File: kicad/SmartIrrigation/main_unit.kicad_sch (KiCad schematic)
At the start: 20 parts, among them J1 RJ45, J2 RJ45, J3 RJ45, J4 RJ45, J5 RJ45, J6 RJ45, J7 Micro_SD_Card, J7 RJ45, J8 RJ45, U6 MT3608

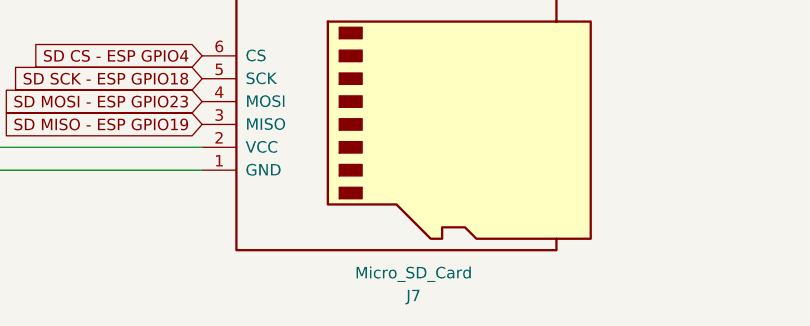
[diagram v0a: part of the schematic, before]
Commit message: added schematics images
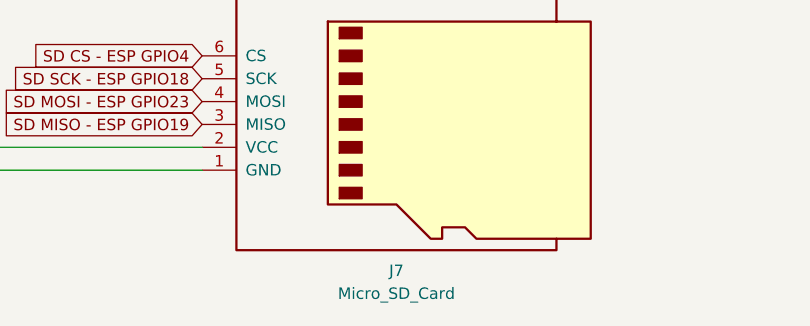
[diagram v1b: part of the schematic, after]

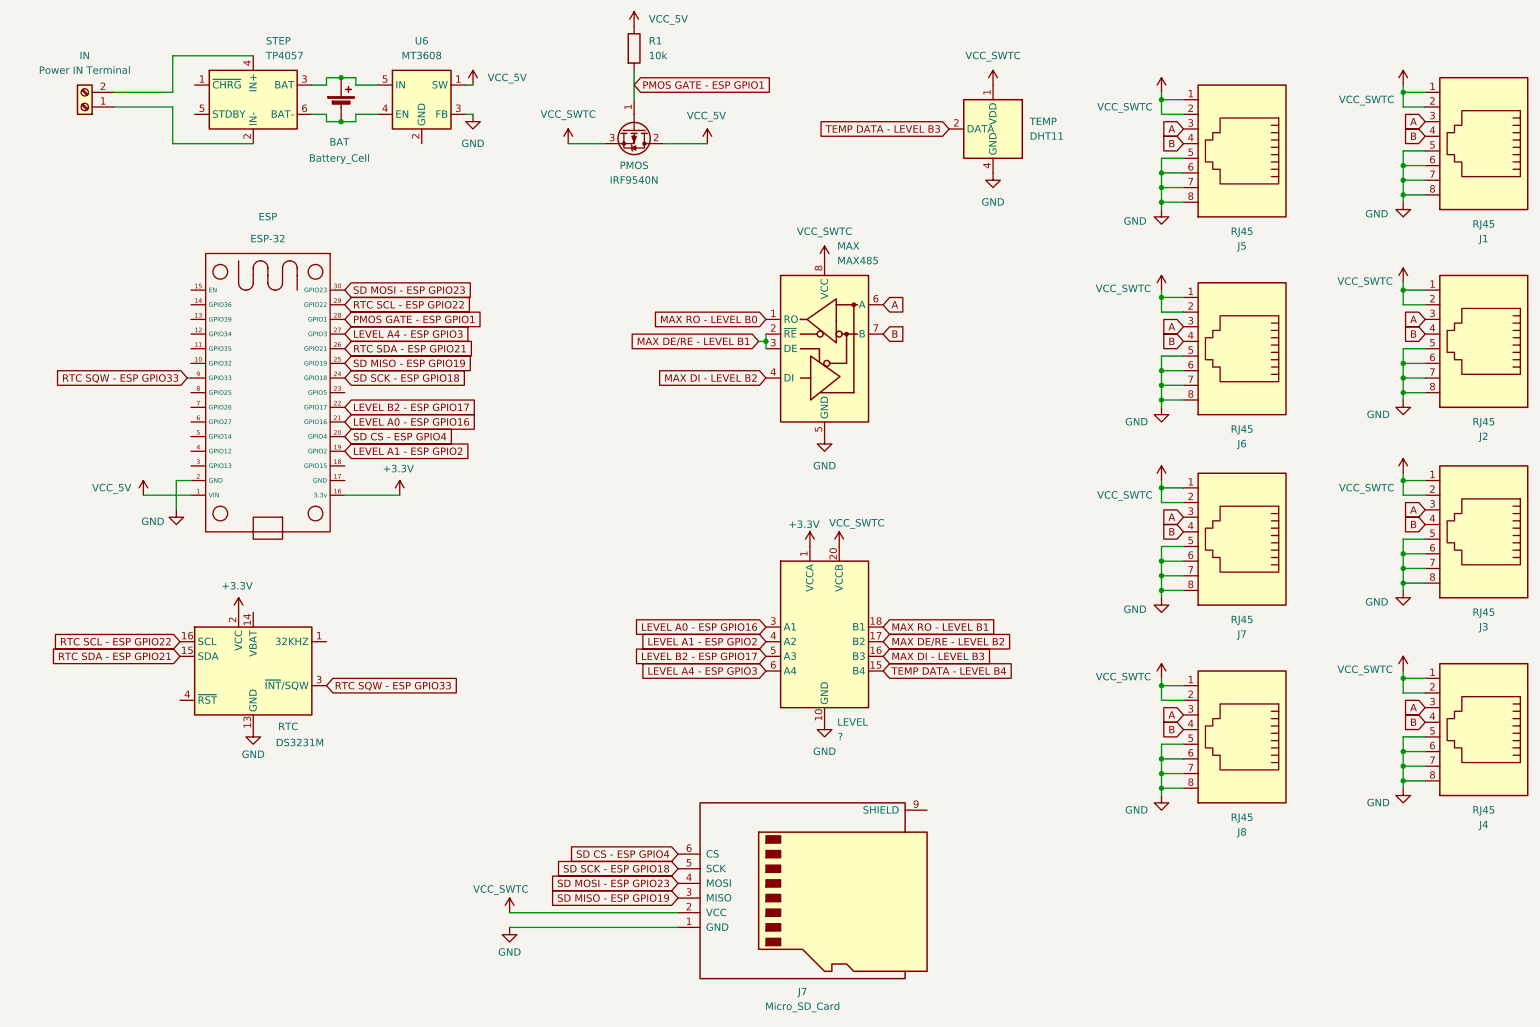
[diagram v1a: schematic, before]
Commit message: new schemes
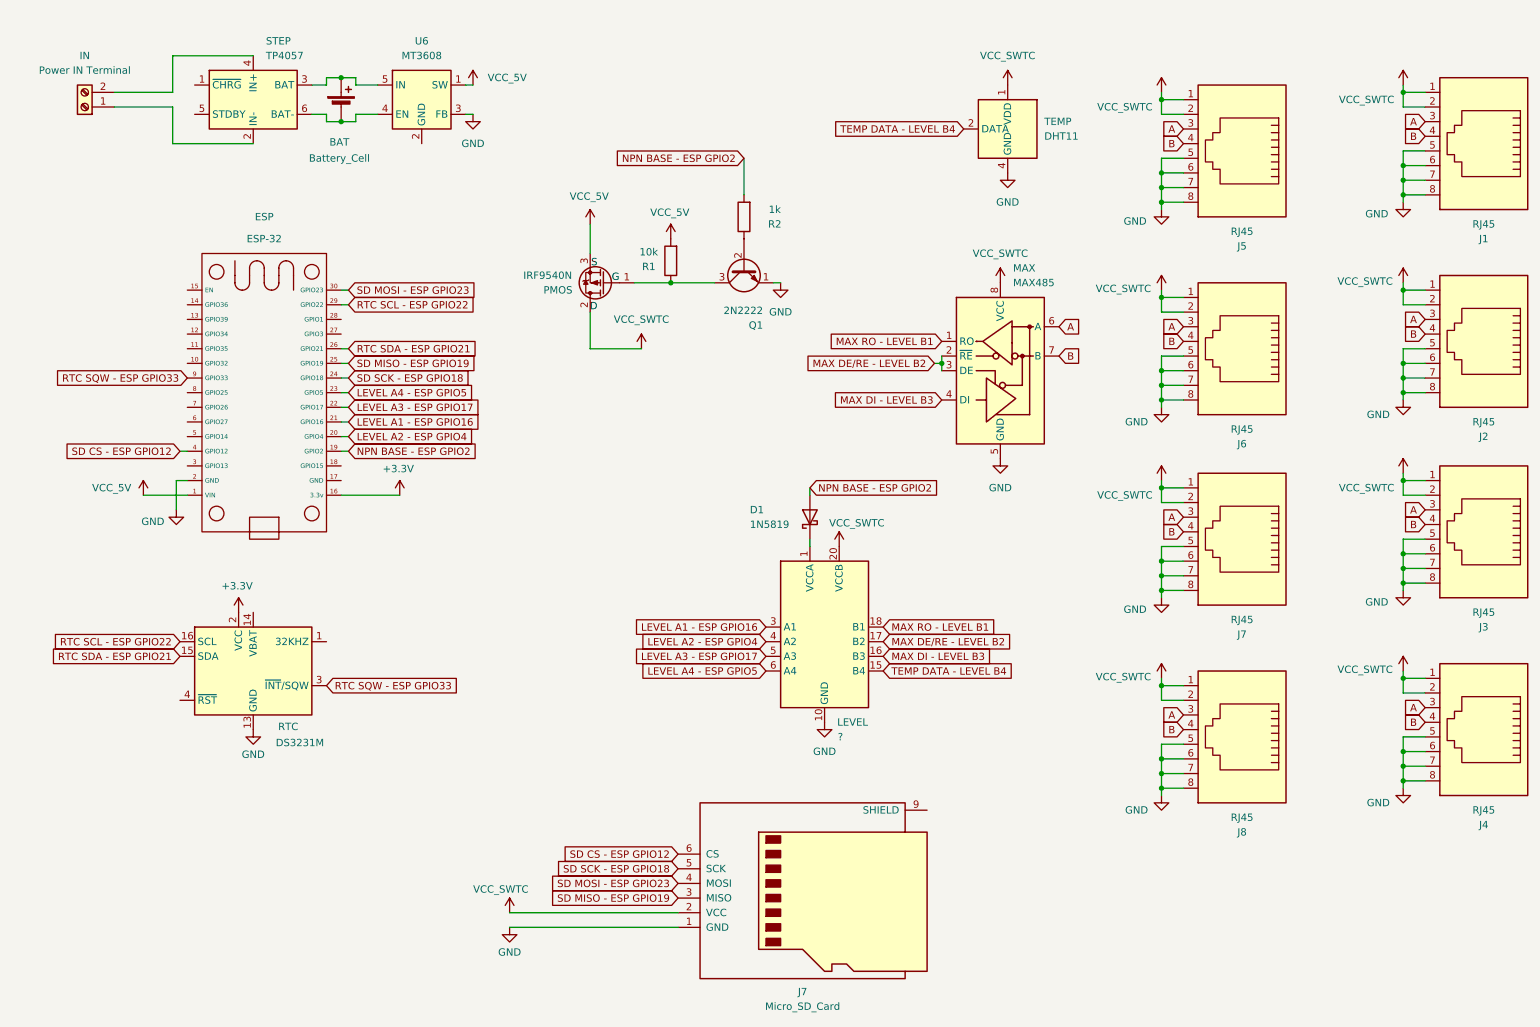
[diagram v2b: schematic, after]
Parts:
- added D1: 1N5819, Diode_THT:D_DO-41_SOD81_P10.16mm_Horizontal, symbol Diode:1N5819
- added Q1: 2N2222, Package_TO_SOT_THT:TO-39-3, symbol Transistor_BJT:2N2219
- added R2: 1k, symbol Device:R
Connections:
- net MAX DE/RE - LEVEL B1 is gone; now on net MAX DE/RE - LEVEL B2: MAX.2 (~{RE}), MAX.3 (DE)
- net MAX DI - LEVEL B2 is gone; now on net MAX DI - LEVEL B3: MAX.4 (DI)
- net MAX RO - LEVEL B0 is gone; now on net MAX RO - LEVEL B1: MAX.1 (RO)
- net TEMP DATA - LEVEL B3 is gone; now on net TEMP DATA - LEVEL B4: TEMP.2 (DATA)
- net +3.3V: no longer LEVEL.1 (VCCA)
- net GND: now also Q1.1 (E)
- net VCC_5V: now also PMOS.3 (S), R1.2; no longer PMOS.2 (D), R1.1
- net VCC_SWTC: now also PMOS.2 (D); no longer PMOS.3 (S)
- net LEVEL A4 - ESP GPIO5: now reaches ESP.23 (GPIO5)
- net LEVEL A4 - ESP GPIO5: now also LEVEL.6 (A4)
- net SD CS - ESP GPIO12: now reaches ESP.4 (GPIO12)
- net SD CS - ESP GPIO12: now also J7.6 (CS)
- net LEVEL A0 - ESP GPIO16 renamed LEVEL A1 - ESP GPIO16
- net LEVEL A1 - ESP GPIO2 renamed LEVEL A2 - ESP GPIO4
- net LEVEL A2 - ESP GPIO4: now also ESP.20 (GPIO4); no longer ESP.19 (GPIO2)
- net LEVEL A4 - ESP GPIO3: no longer names the net of ESP.27 (GPIO3)
- net LEVEL A4 - ESP GPIO3: no longer LEVEL.6 (A4)
- net LEVEL B2 - ESP GPIO17 renamed LEVEL A3 - ESP GPIO17
- removed net PMOS GATE - ESP GPIO1: ESP.28 (GPIO1), PMOS.1 (G), R1.2
- removed net SD CS - ESP GPIO4: ESP.20 (GPIO4), J7.6 (CS)
- new net: D1.1 (K), LEVEL.1 (VCCA)
- new net: PMOS.1 (G), Q1.3 (C), R1.1
- new net: Q1.2 (B), R2.1
- new net NPN BASE - ESP GPIO2: D1.2 (A), ESP.19 (GPIO2), R2.2
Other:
- moved on the sheet: ESP, MAX, PMOS, R1, TEMP
